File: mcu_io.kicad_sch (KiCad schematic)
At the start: 16 parts, among them U3 SiWG917Y, U9 PCAL6408AHK

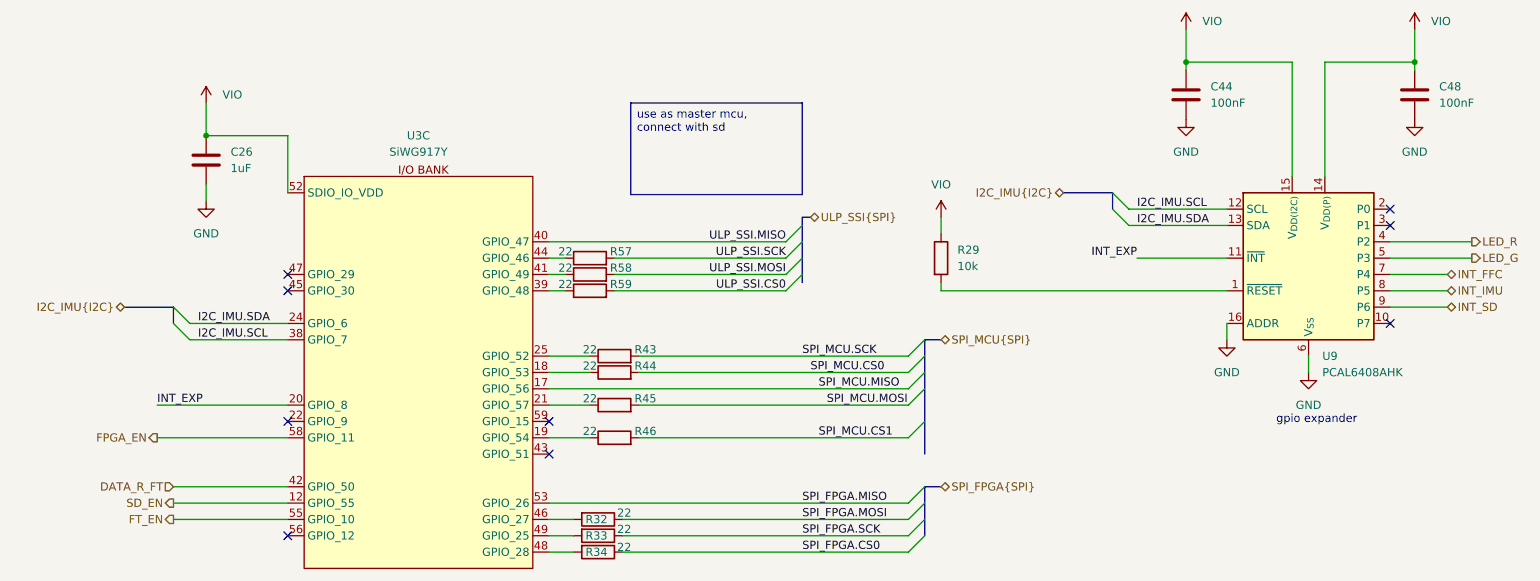
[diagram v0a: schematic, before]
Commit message: Comments on layout
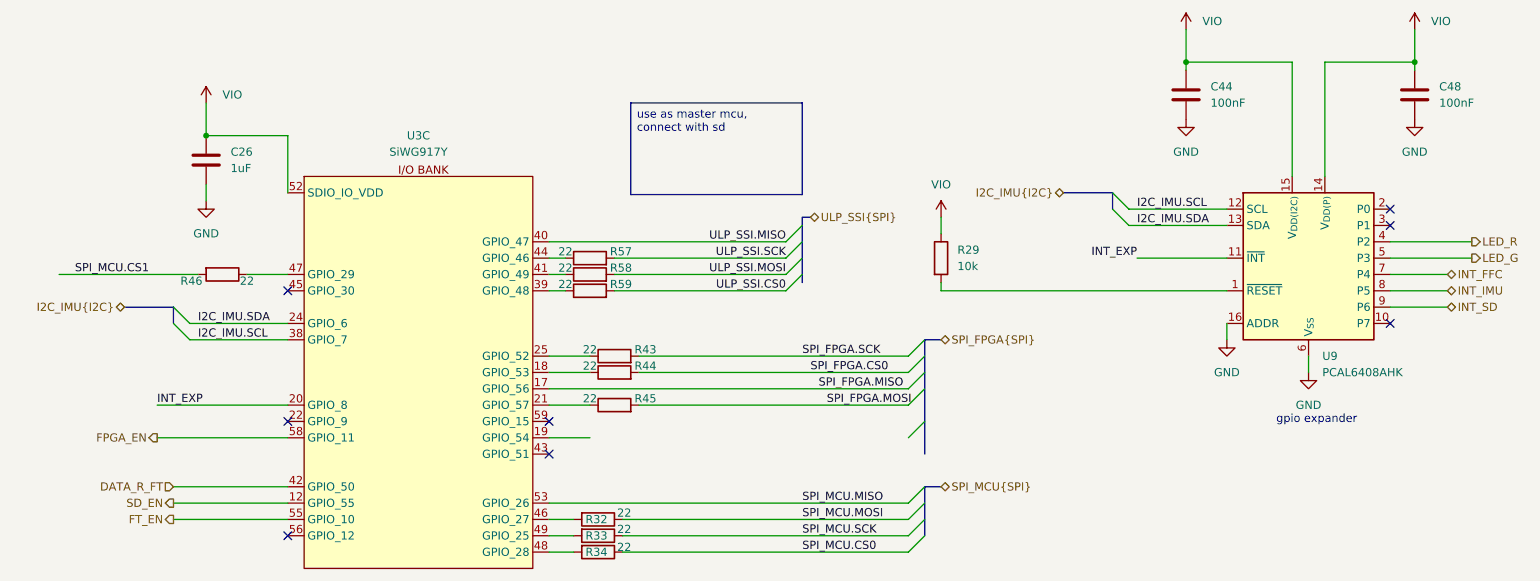
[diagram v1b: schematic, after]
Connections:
- net SPI_FPGA.CS0: now also R44.2; no longer R34.1
- net SPI_FPGA.MISO: now also U3.17 (GPIO_56); no longer U3.53 (GPIO_26)
- net SPI_FPGA.MOSI: now also R45.2; no longer R32.1
- net SPI_FPGA.SCK: now also R43.2; no longer R33.1
- net SPI_MCU.CS0: now also R34.1; no longer R44.2
- net SPI_MCU.MISO: now also U3.53 (GPIO_26); no longer U3.17 (GPIO_56)
- net SPI_MCU.MOSI: now also R32.1; no longer R45.2
- net SPI_MCU.SCK: now also R33.1; no longer R43.2
- net at R46.1: now also U3.47 (GPIO_29); no longer U3.19 (GPIO_54)
- no-connect marks 9 -> 8
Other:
- moved on the sheet: R46
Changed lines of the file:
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@@
-	)
-	(no_connect
-		(at 55.88 73.66)
 	)
 	(no_connect
@@
 	(wire
 		(pts
+			(xy 49.53 73.66) (xy 55.88 73.66)
+		)
+		(stroke
+			(width 0)
+			(type default)
+		)
+	)
+	(wire
+		(pts
 			(xy 96.52 71.12) (xy 99.06 71.12)
 		)
@@
 	(wire
 		(pts
-			(xy 110.49 99.06) (xy 152.4 99.06)
+			(xy 41.91 73.66) (xy 20.32 73.66)
 		)
 		(stroke
@@
 	)
 	(label "SPI_MCU.CS0"
-		(at 137.16 88.9 0)
+		(at 135.89 116.84 0)
 		(effects
 			(font
@@
 	)
 	(label "SPI_MCU.MOSI"
-		(at 139.7 93.98 0)
+		(at 135.89 111.76 0)
 		(effects
 			(font
@@
 	)
 	(label "SPI_FPGA.SCK"
-		(at 135.89 114.3 0)
+		(at 135.89 86.36 0)
 		(effects
 			(font
@@
 	)
 	(label "SPI_MCU.CS1"
-		(at 138.43 99.06 0)
-		(effects
-			(font
-				(size 1.27 1.27)
-			)
-			(justify left bottom)
+		(at 34.29 73.66 180)
+		(effects
+			(font
+				(size 1.27 1.27)
+			)
+			(justify right bottom)
 		)
 	)
@@
 	)
 	(label "SPI_FPGA.CS0"
-		(at 135.89 116.84 0)
+		(at 137.16 88.9 0)
 		(effects
 			(font
@@
 	)
 	(label "SPI_MCU.MISO"
-		(at 138.43 91.44 0)
+		(at 135.89 109.22 0)
 		(effects
 			(font
@@
 	)
 	(label "SPI_FPGA.MOSI"
-		(at 135.89 111.76 0)
+		(at 139.7 93.98 0)
 		(effects
 			(font
@@
 	)
 	(label "SPI_FPGA.MISO"
-		(at 135.89 109.22 0)
+		(at 138.43 91.44 0)
 		(effects
 			(font
@@
 	)
 	(label "SPI_MCU.SCK"
-		(at 135.89 86.36 0)
+		(at 135.89 114.3 0)
 		(effects
 			(font
@@
 	(hierarchical_label "SPI_MCU{SPI}"
 		(shape bidirectional)
-		(at 157.48 83.82 0)
+		(at 157.48 106.68 0)
 		(effects
 			(font
@@
 	(hierarchical_label "SPI_FPGA{SPI}"
 		(shape bidirectional)
-		(at 157.48 106.68 0)
+		(at 157.48 83.82 0)
 		(effects
 			(font
@@
 	(symbol
 		(lib_id "#dzdb:g_res/R-22-0201")
-		(at 106.68 99.06 90)
+		(at 45.72 73.66 270)
 		(unit 1)
 		(body_style 1)
@@
 		(dnp no)
 		(property "Reference" "R46"
-			(at 111.506 98.044 90)
+			(at 40.894 74.676 90)
 			(show_name no)
 			(do_not_autoplace no)
@@
 		)
 		(property "Value" "22"
-			(at 102.87 98.044 90)
+			(at 49.53 74.676 90)
 			(show_name no)
 			(do_not_autoplace no)
@@
 		)
 		(property "Footprint" "Resistor_SMD:R_0201_0603Metric"
-			(at 106.68 100.838 90)
+			(at 45.72 71.882 90)
 			(hide yes)
 			(show_name no)
@@
 		)
 		(property "Datasheet" "https://industrial.panasonic.com/ww/products/pt/general-purpose-chip-resistors/models/ERJ1GJF22R0C"
-			(at 106.68 99.06 0)
+			(at 45.72 73.66 0)
 			(hide yes)
 			(show_name no)
@@
 		)
 		(property "Description" "Res 22Ω 0201 0.05W Thick Film ±1%"
-			(at 106.68 99.06 0)
+			(at 45.72 73.66 0)
 			(hide yes)
 			(show_name no)
@@
 		)
 		(property "Power" "0.05W"
-			(at 106.68 99.06 0)
+			(at 45.72 73.66 0)
 			(hide yes)
 			(show_name no)
@@
 		)
 		(property "Tolerance" "1%"
-			(at 106.68 99.06 0)
+			(at 45.72 73.66 0)
 			(hide yes)
 			(show_name no)
@@
 		)
 		(property "Resistance" "22"
-			(at 106.68 99.06 0)
+			(at 45.72 73.66 0)
 			(hide yes)
 			(show_name no)
@@
 		)
 		(property "SPN" "667-ERJ-1GJF22R0C"
-			(at 106.68 99.06 0)
+			(at 45.72 73.66 0)
 			(hide yes)
 			(show_name no)
@@
 		)
 		(property "LCSC" "C20021234"
-			(at 106.68 99.06 0)
+			(at 45.72 73.66 0)
 			(hide yes)
 			(show_name no)
@@
 		)
 		(property "MPN" "ERJ-1GJF22R0C"
-			(at 106.68 99.06 0)
+			(at 45.72 73.66 0)
 			(hide yes)
 			(show_name no)
@@
 		)
 		(property "Supplier" "Mouser"
-			(at 106.68 99.06 0)
+			(at 45.72 73.66 0)
 			(hide yes)
 			(show_name no)
@@
 		)
 		(property "Manufacturer" "Panasonic"
-			(at 106.68 99.06 0)
+			(at 45.72 73.66 0)
 			(hide yes)
 			(show_name no)
@@
 		)
 		(property "IPN" "R-22-0201"
-			(at 106.68 99.06 0)
+			(at 45.72 73.66 0)
 			(hide yes)
 			(show_name no)
@@
 		)
 		(property "Material" "Thick Film"
-			(at 106.68 99.06 0)
+			(at 45.72 73.66 0)
 			(hide yes)
 			(show_name no)
@@
 		)
 		(property "Comment" "lifecycle=Active;note=AEC-Q200 compliant;TCR=±200ppm/°C"
-			(at 106.68 99.06 0)
-			(hide yes)
-			(show_name no)
+			(at 45.72 73.66 0)
+			(hide yes)
+			(show_name no)
